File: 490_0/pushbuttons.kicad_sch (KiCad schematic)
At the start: 5 parts, among them SW1 SW_Push0, SW2 SW_Push1, SW3 SW_Push2, SW4 SW_Push3, SW5 SW_Push4

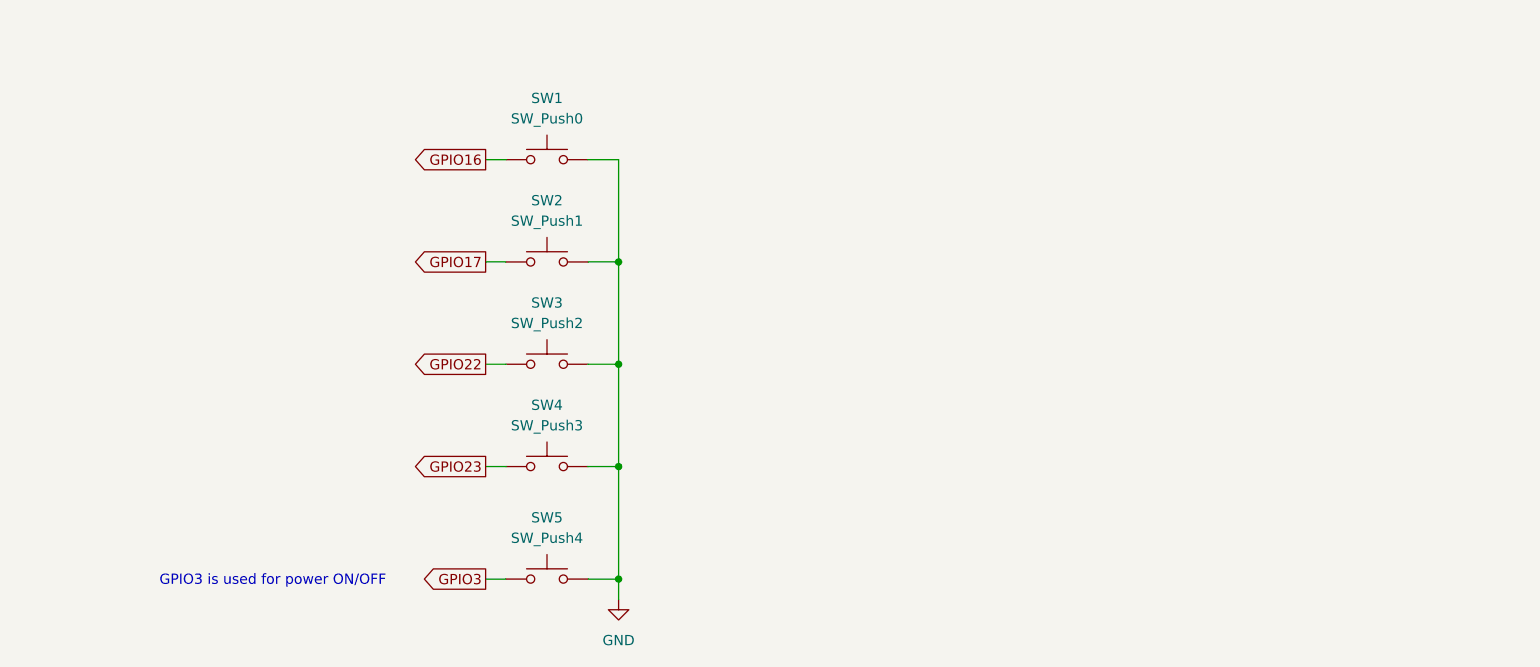
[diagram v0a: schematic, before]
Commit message: Fixed buttons
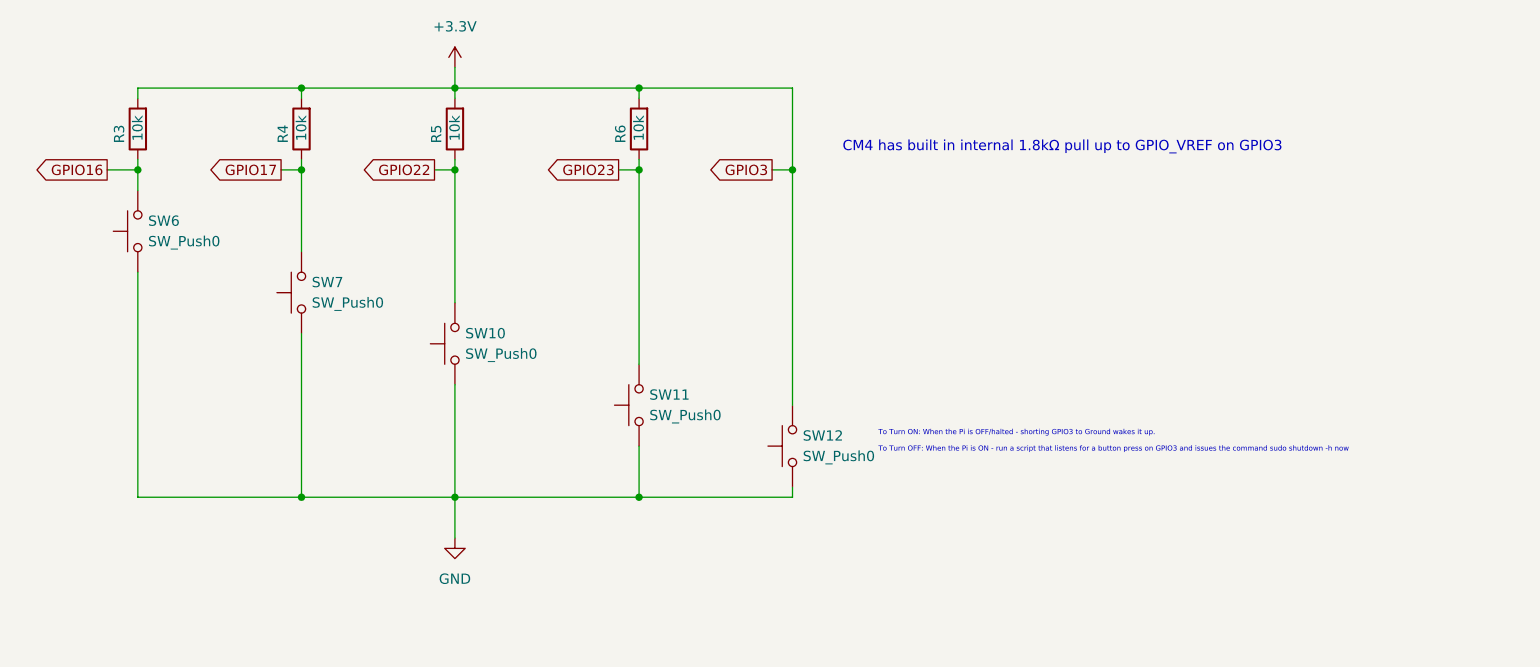
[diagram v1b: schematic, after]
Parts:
- removed SW1: SW_Push0, symbol Switch:SW_Push
- removed SW2: SW_Push1, symbol Switch:SW_Push
- removed SW3: SW_Push2, symbol Switch:SW_Push
- removed SW4: SW_Push3, symbol Switch:SW_Push
- removed SW5: SW_Push4, symbol Switch:SW_Push
- added R3, R4, R5, R6: 10k, symbol Device:R
- added SW10, SW11, SW12, SW6, SW7: SW_Push0, symbol Switch:SW_Push
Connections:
- net GND: now also SW10.1, SW11.1, SW12.1, SW6.1, SW7.1
- net GPIO16: now also R3.1, SW6.2
- net GPIO17: now also R4.1, SW7.2
- net GPIO22: now also R5.1, SW10.2
- net GPIO23: now also R6.1, SW11.2
- new net +3.3V: R3.2, R4.2, R5.2, R6.2, SW12.2
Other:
- note added: "CM4 has built in internal 1.8kΩ pull up to GPIO_VREF on GPIO3"
- note added: "To Turn ON: When the Pi is OFF/halted - shorting GPIO3 to Ground wakes it up. To Turn OFF: When the Pi is ON - run a script that listens for a button press on GPIO3 and issues the command sudo shutdown -h now"
- note removed: "GPIO3 is used for power ON/OFF"
